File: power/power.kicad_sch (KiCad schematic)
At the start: 25 parts, among them J0 JST-XH conn, J1 BAT-conn, J10 A2212 conn, J11 BAT-conn, J12 A2212 conn, J13 PWM Conn, J14 A2212 conn, J15 BAT-conn, J16 A2212 conn, J17 PWM Conn, J18 A2212 conn, J19 ESP_OUT, J2 JST-XH conn, J20 ESP_IN, J3 BAT-conn, J4 A2212 conn, J5 PWM Conn, J6 A2212 conn, J7 BAT-conn, J8 A2212 conn, J9 PWM Conn

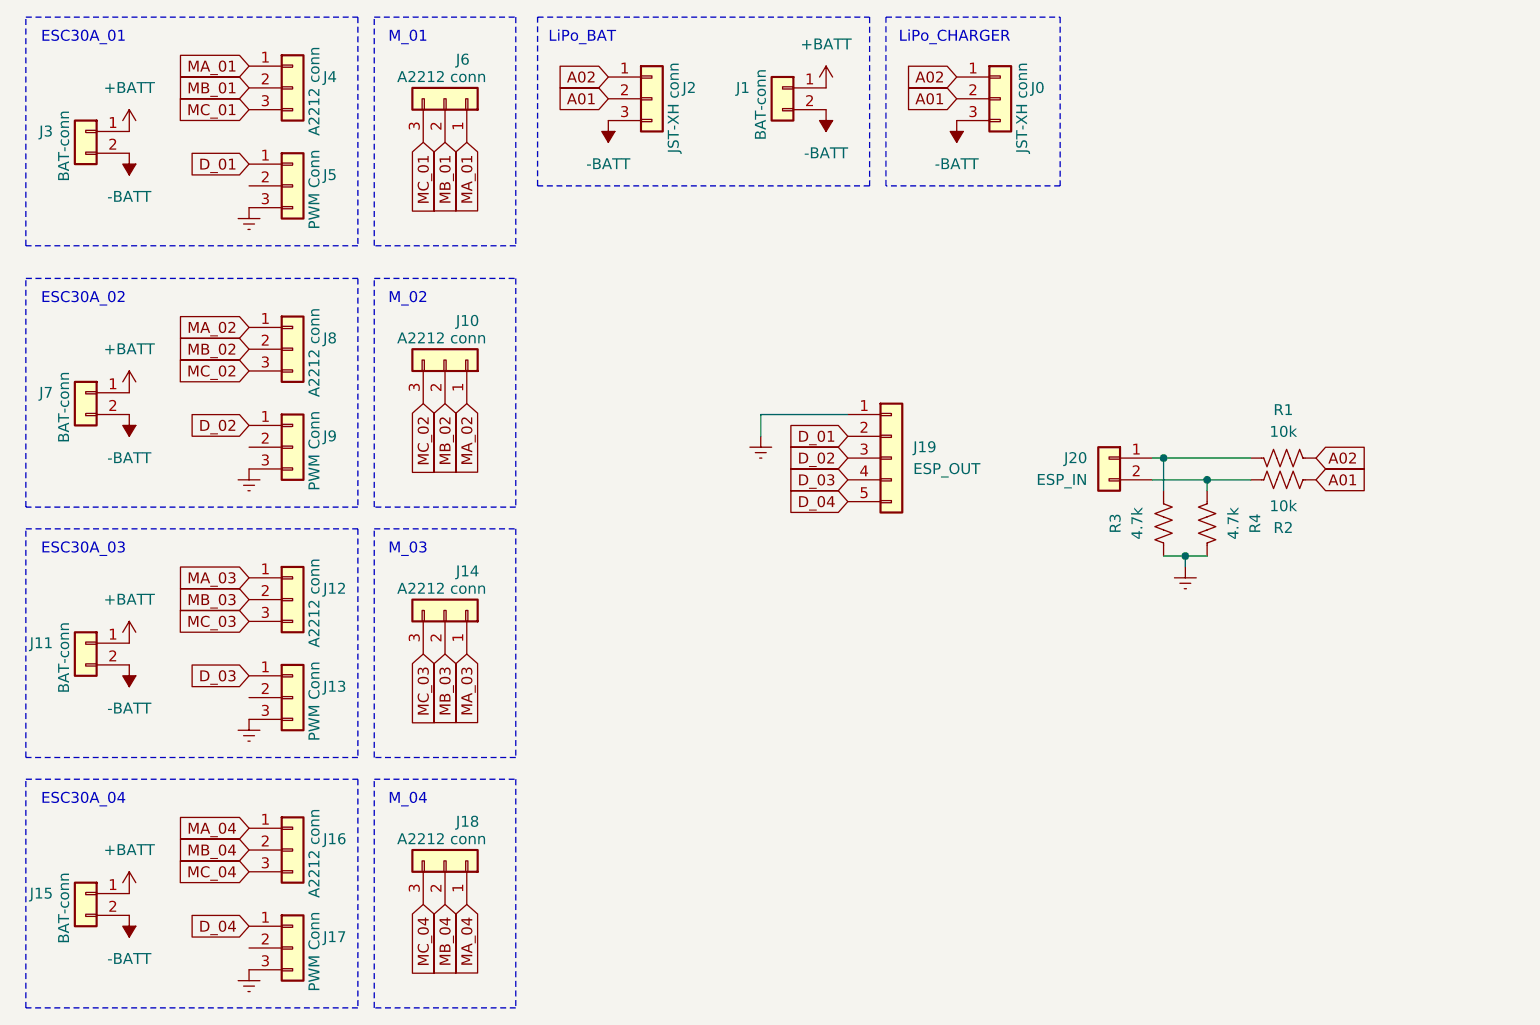
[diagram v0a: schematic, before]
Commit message: chore (electronic | power): update electronic subprojects
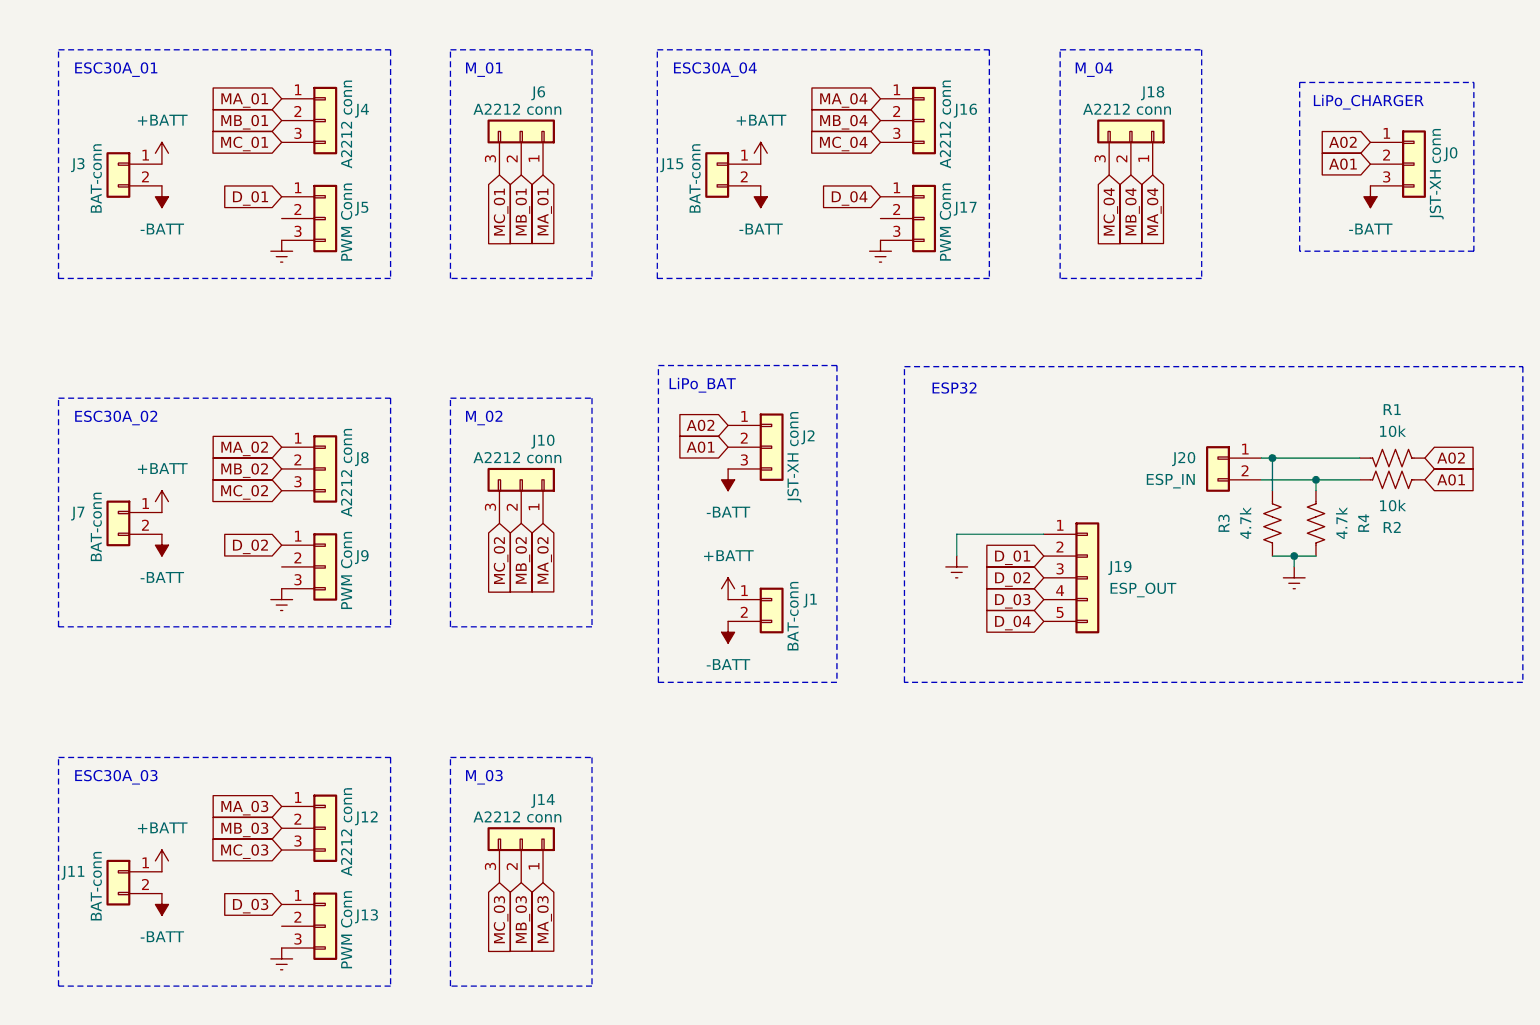
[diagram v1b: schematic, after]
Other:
- note added: "ESP32"
- title: (none) -> Esquematico 2 de la plataforma
- moved on the sheet: J0, J1, J10, J11, J12, J13, J14, J15, J16, J17, J18, J19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
